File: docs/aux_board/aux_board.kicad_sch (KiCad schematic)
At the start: 16 parts, among them J1 SPI et GPIO interfaces, J2 Encoder Interface, U3 LS7366R-S, Y1 40 MHz

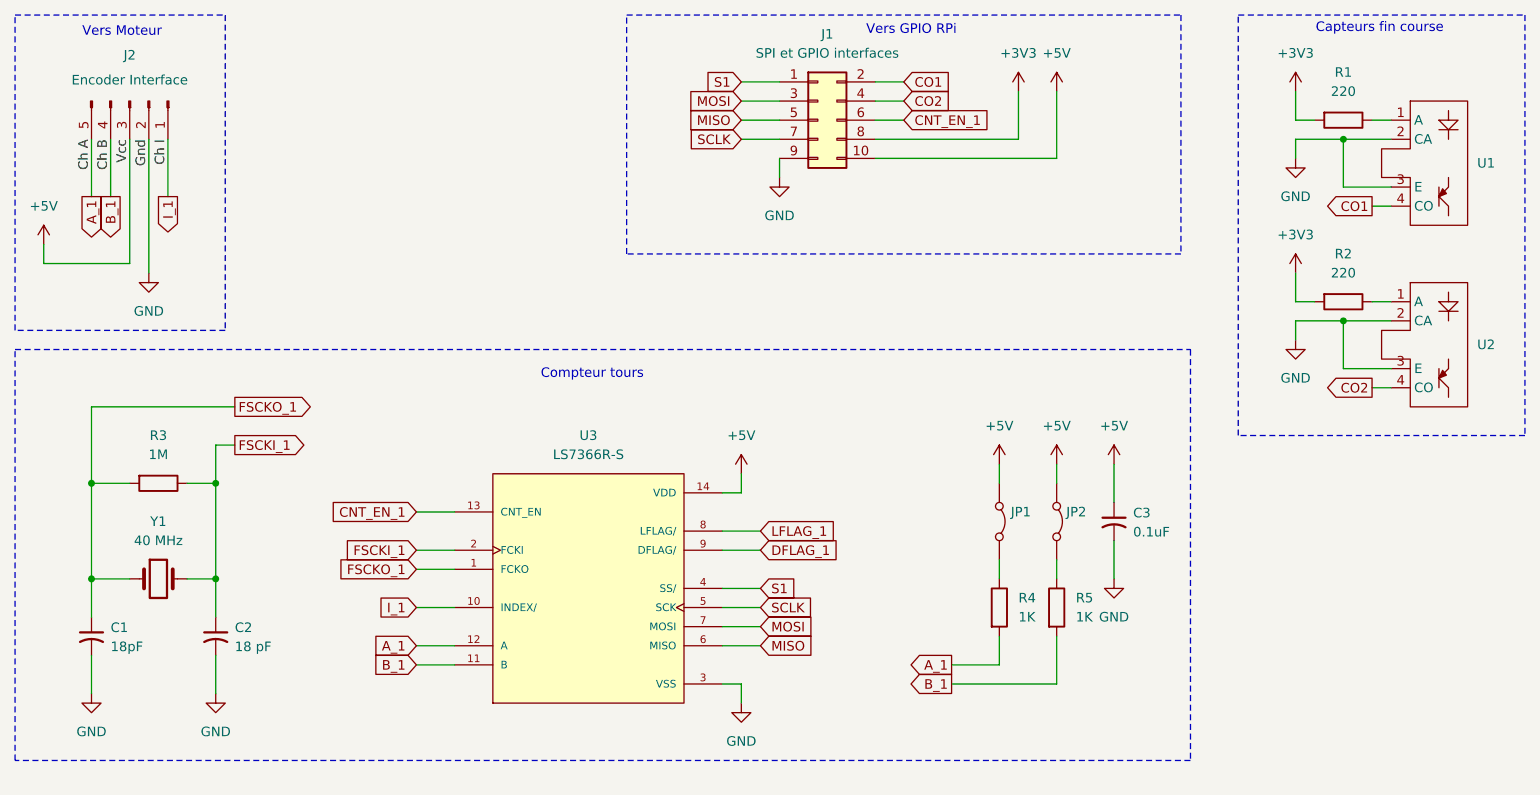
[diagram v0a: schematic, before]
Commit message: pcb
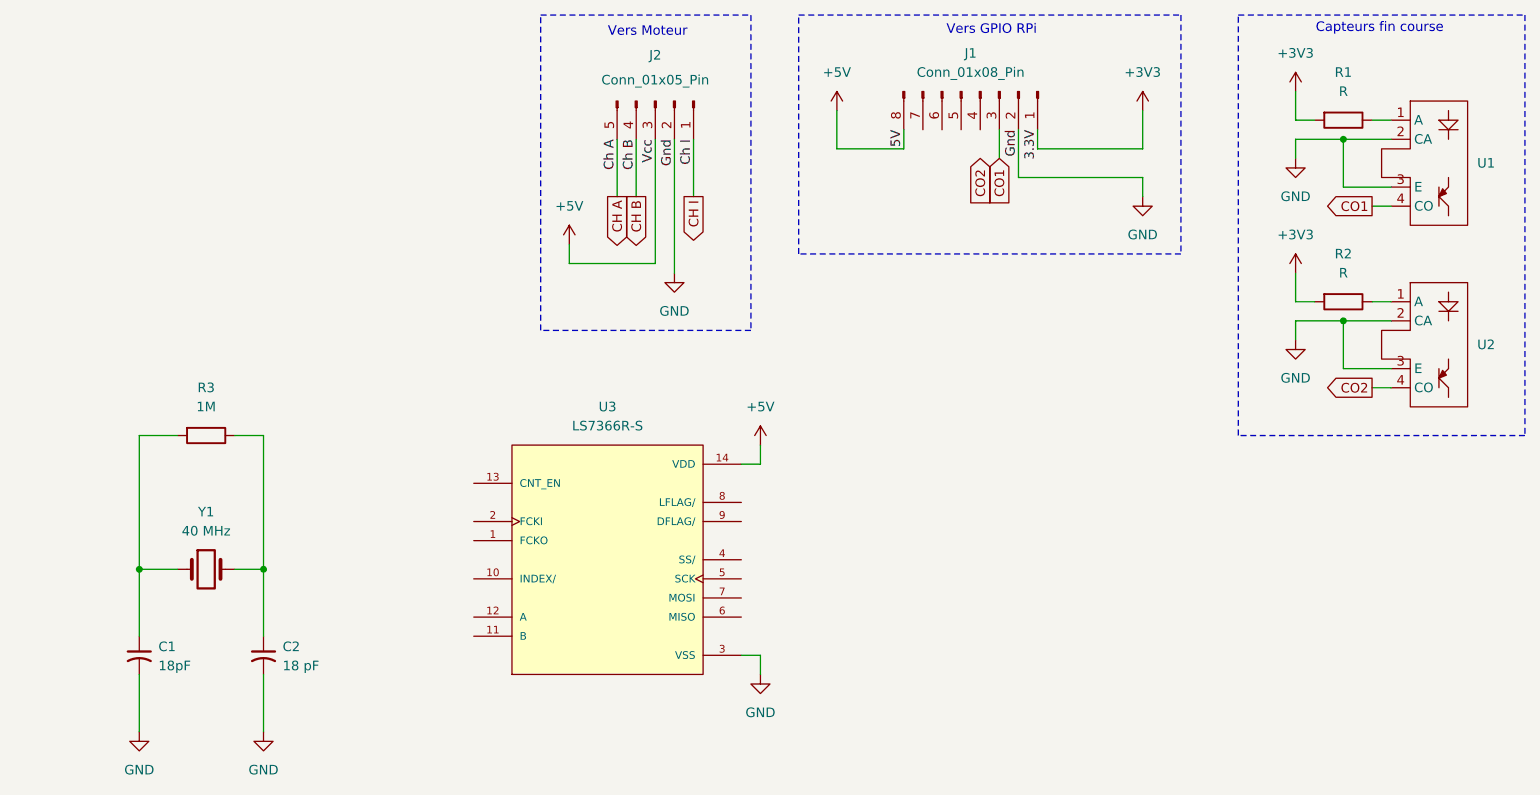
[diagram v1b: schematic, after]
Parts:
- removed C3: 0.1uF, symbol Device:C_Small_US
- removed J1: SPI et GPIO interfaces, Connector_PinHeader_2.54mm:PinHeader_2x05_P2.54mm_Vertical, symbol Connector_Generic:Conn_02x05_Odd_Even
- removed JP1, JP2: Jumper_2_Bridged, symbol Jumper:Jumper_2_Bridged
- removed R4, R5: 1K, symbol Device:R
- added J1: Conn_01x08_Pin, symbol Connector:Conn_01x08_Pin
- J2: value Encoder Interface -> Conn_01x05_Pin; footprint Connector_PinHeader_2.54mm:PinHeader_1x05_P2.54mm_Vertical -> (none)
- R1, R2: value 220 -> R
- U3: footprint Package_SO:SOIC-14_3.9x8.7mm_P1.27mm -> LS7366R-S:SOIC127P600X175-14N
- Y1: footprint Crystal:Crystal_SMD_2520-4Pin_2.5x2.0mm -> (none)
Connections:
- net +3V3: now also J1.1 (Pin_1)
- net +5V: now also J1.8 (Pin_8)
- net CO1: now also J1.3 (Pin_3)
- net GND: now also J1.2 (Pin_2)
- net A_1: no longer names the net of U3.12 (A)
- net A_1: no longer J2.5 (Pin_5)
- net B_1: no longer names the net of U3.11 (B)
- net B_1: no longer J2.4 (Pin_4)
- net CNT_EN_1: no longer names the net of U3.13 (CNT_EN)
- net DFLAG_1: no longer names the net of U3.9 (DFLAG/)
- net FSCKI_1: no longer names the net of C2.1, R3.1, Y1.2
- net FSCKI_1: no longer U3.2 (FCKI)
- net FSCKO_1: no longer names the net of C1.1, R3.2, Y1.1
- net FSCKO_1: no longer U3.1 (FCKO)
- net I_1: no longer names the net of U3.10 (INDEX/)
- net I_1: no longer J2.1 (Pin_1)
- net LFLAG_1: no longer names the net of U3.8 (LFLAG/)
- net MISO: no longer names the net of U3.6 (MISO)
- net MOSI: no longer names the net of U3.7 (MOSI)
- net S1: no longer names the net of U3.4 (SS/)
- net SCLK: no longer names the net of U3.5 (SCK)
- new net CH A: J2.5 (Pin_5)
- new net CH B: J2.4 (Pin_4)
- new net CH I: J2.1 (Pin_1)
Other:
- note removed: "Compteur tours"
- moved on the sheet: C1, C2, J2, R3, U3, Y1
